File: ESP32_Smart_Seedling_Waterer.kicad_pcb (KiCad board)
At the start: 2 copper layers, 84.3 x 51.3 mm, 23 parts, among them J1 Solenoid_12V, J2 AM2302 ~ DHT22, J3 Barrel_Jack_Switch, K1 SRD-05VDC-SL-C, Q1 PN2222A, Q2 PN2222A, SW1 SW_Push, SW3 SW_SPST, U1 LM7805_TO220, U2 ESP32-C3 SuperMini

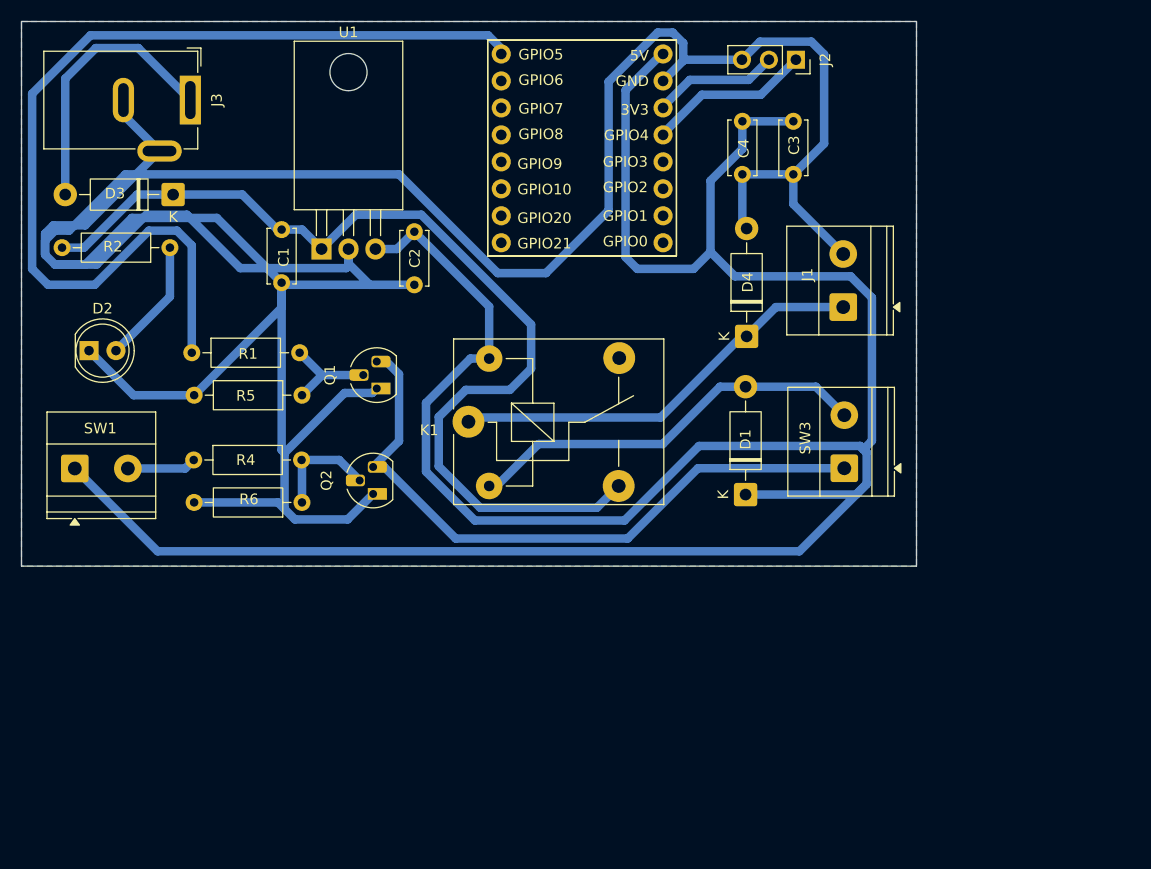
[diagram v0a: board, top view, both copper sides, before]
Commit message: 9.3.2026
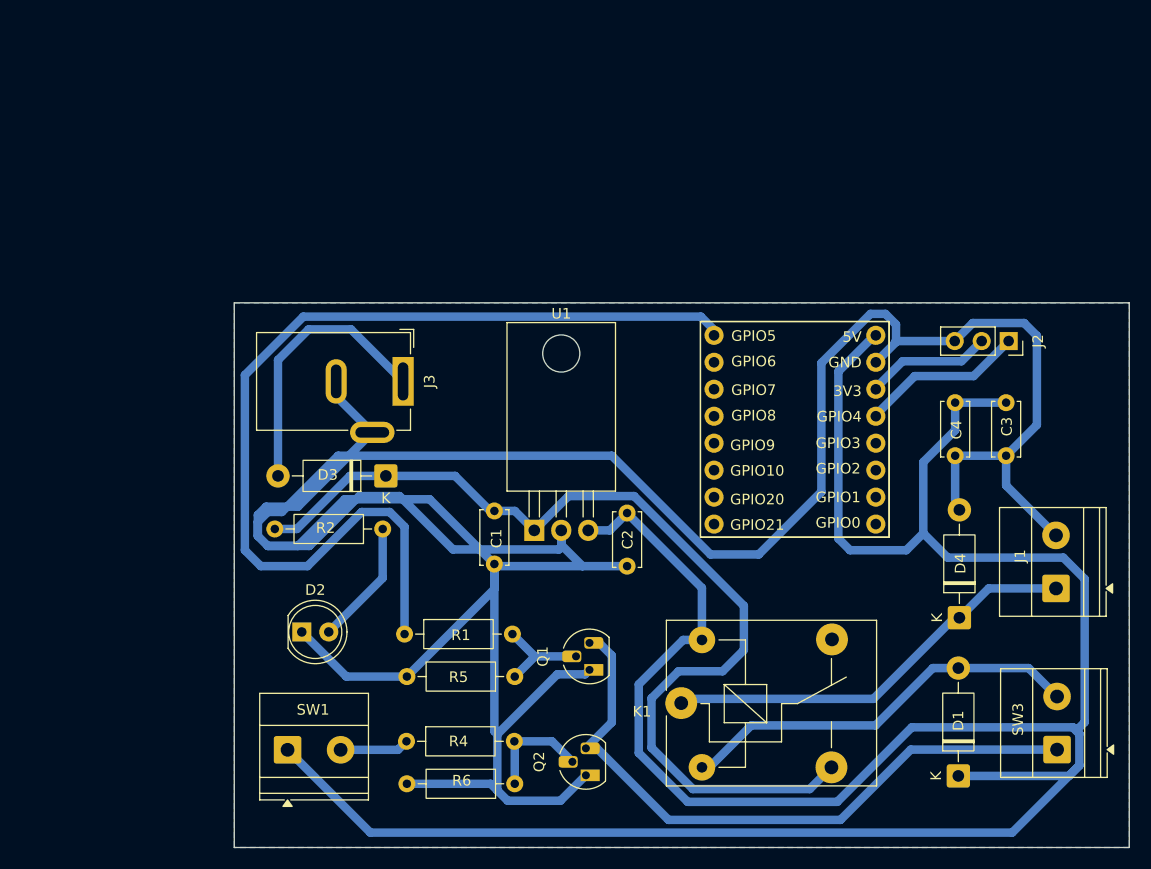
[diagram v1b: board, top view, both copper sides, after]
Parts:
- moved D4 33.2 mm to (164.7, 100.3)
- moved U2 33.2 mm to (149.2, 80.2)
- moved C2 33.2 mm to (133.4, 90.4)
- moved D3 33.2 mm to (110.7, 86.9)
- moved J3 33.2 mm to (112.3, 78.0)
- moved Q1 33.2 mm to (129.9, 105.2)
- moved Q2 33.2 mm to (129.6, 115.1)
- moved R1 33.2 mm to (112.5, 101.8)
- moved R2 33.2 mm to (110.4, 91.9)
- moved R5 33.2 mm to (122.9, 105.8)
- moved R6 33.2 mm to (122.9, 115.9)
- moved U1 33.2 mm to (124.7, 92.0)
- moved C1 33.2 mm to (120.9, 90.2)
- moved C3 33.2 mm to (169.1, 80.0)
- moved C4 33.2 mm to (164.3, 80.0)
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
